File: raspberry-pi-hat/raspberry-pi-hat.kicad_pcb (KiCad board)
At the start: 2 copper layers, 58.5 x 66.5 mm, 31 parts, among them J1 IR_IN_JACK, J2 IR_OUT_JACK, J3 ADC0_JACK, J4 ADC1_JACK, J5 IR_IN_JMP, J6 IR_OUT_JMP, P1 RPi-GPIO, Q1 IRLML2803TRPBF, U1 MCP3204, U2 74AC86

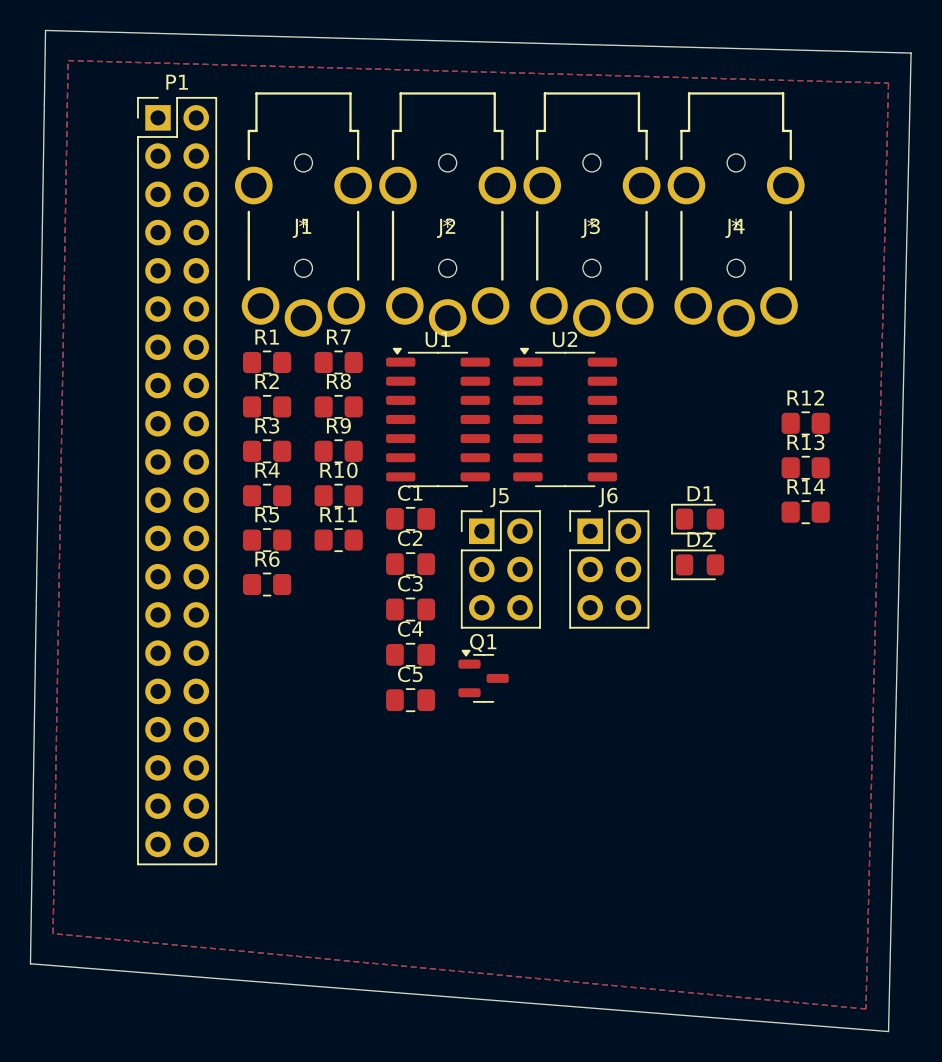
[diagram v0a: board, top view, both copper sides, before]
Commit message: pcb layout
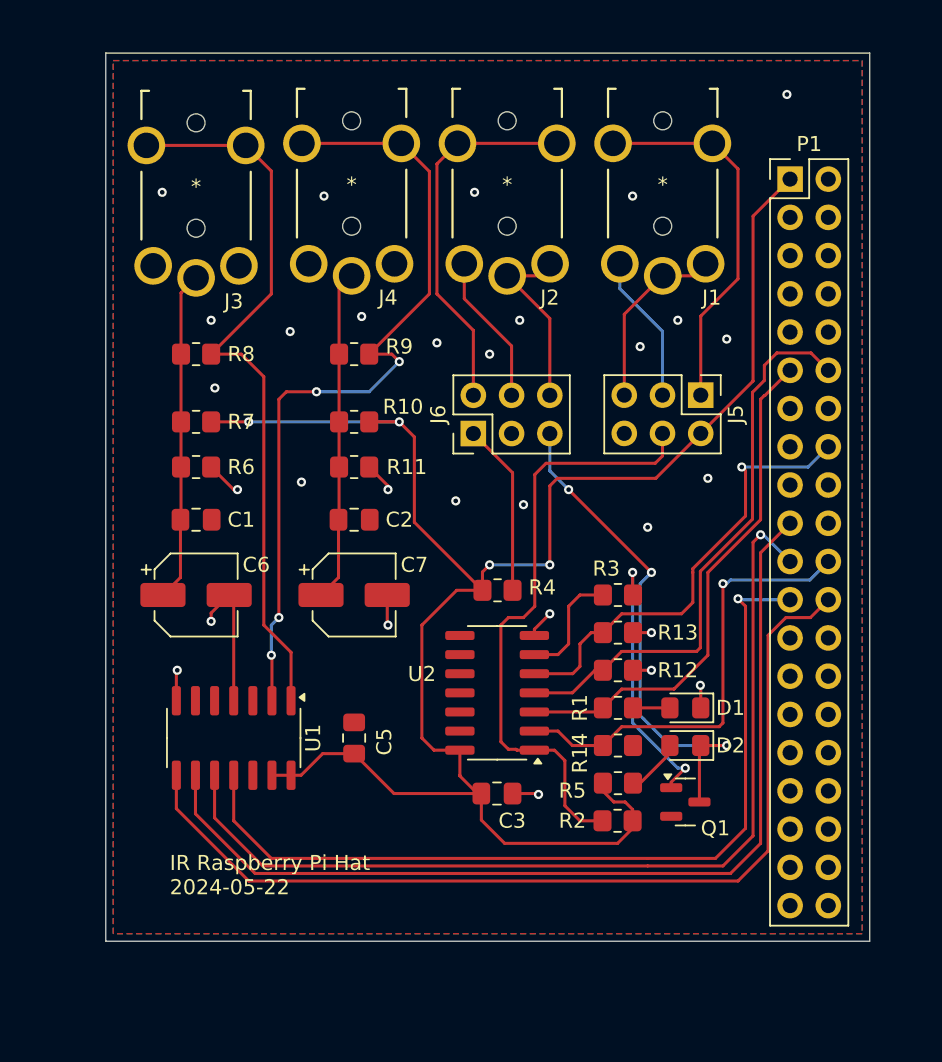
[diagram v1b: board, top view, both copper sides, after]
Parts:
- removed C4: 0.1uF, Capacitor_SMD:C_0805_2012Metric_Pad1.18x1.45mm_HandSolder
- added C6: 100uF, Capacitor_SMD:CP_Elec_5x5.3, F.Cu at (53.5, 86.5)
- added C7: 100uF, Capacitor_SMD:CP_Elec_5x5.3, F.Cu at (64.0, 86.5)
- moved P1 42.2 mm to (93.0, 58.9)
- moved R2 36.0 mm to (81.5, 101.5), turned to 180 degrees
- moved R1 32.7 mm to (81.5, 94.0)
- moved R5 28.4 mm to (81.5, 99.0), turned to 180 degrees
- moved J3 26.4 mm to (53.5, 59.4)
- moved J4 25.7 mm to (63.8, 59.2)
- moved R3 25.2 mm to (81.5, 86.5)
- moved U1 25.1 mm to (56.0, 96.0), turned to -90 degrees
- moved J1 24.0 mm to (84.5, 59.2)
- moved R12 20.6 mm to (81.5, 91.5), turned to 180 degrees
- moved R14 19.9 mm to (81.5, 96.5), turned to 180 degrees
- moved U2 18.7 mm to (73.5, 93.0), turned to 180 degrees
- moved J5 17.1 mm to (87.0, 73.2), turned to -90 degrees
- moved R13 16.6 mm to (81.5, 89.0), turned to 180 degrees
- moved R4 16.5 mm to (73.5, 86.2), turned to 180 degrees
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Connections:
- C1 pad 2: <NO NET> -> GND
- C2 pad 2: <NO NET> -> GND
- C3 pad 2: <NO NET> -> GND
- C5 pad 2: <NO NET> -> GND
- D1 pad 1: <NO NET> -> GND
- J1 pad R2: Net-(J5-Pin_1) -> Net-(J5-Pin_5)
- J1 pad S: Net-(J5-Pin_1) -> Net-(J5-Pin_5)
- J1 pad T: Net-(J5-Pin_5) -> Net-(J5-Pin_1)
- J5 pad 6: <NO NET> -> GND
- J6 pad 3: Net-(D2-K) -> unconnected-(J6-Pin_3-Pad3)
- P1 pad 25: <NO NET> -> GND
- P1 pad 39: <NO NET> -> GND
- P1 pad 9: <NO NET> -> GND
- Q1 pad 2: <NO NET> -> GND
- R11 pad 1: <NO NET> -> GND
- R12 pad 1: <NO NET> -> GND
- R13 pad 1: <NO NET> -> GND
- R14 pad 1: <NO NET> -> GND
- R6 pad 1: <NO NET> -> GND
- U1 pad 12: <NO NET> -> GND
- U1 pad 3: <NO NET> -> GND
- U1 pad 4: <NO NET> -> GND
- U1 pad 7: <NO NET> -> GND
- U2 pad 10: <NO NET> -> GND
- U2 pad 12: <NO NET> -> GND
- U2 pad 13: <NO NET> -> GND
- U2 pad 7: <NO NET> -> GND
- U2 pad 9: <NO NET> -> GND
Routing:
- net +3.3V: track 0.00 -> 121.6 mm, vias 0 -> 4
- net /MOSI: track 0.00 -> 64.6 mm
- net /MISO: track 0.00 -> 63.7 mm, vias 0 -> 1
- net /ADC_CS: track 0.00 -> 63.6 mm
- net /SCLK: track 0.00 -> 57.8 mm, vias 0 -> 1
- net /ADC_CH1: track 0.00 -> 54.5 mm, vias 0 -> 4
- net /ADC_CH0: track 0.00 -> 49.2 mm
- net Net-(J5-Pin_4): track 0.00 -> 40.4 mm
- net /IR_OUT: track 0.00 -> 37.9 mm
- net /IR_IN: track 0.00 -> 34.3 mm
- net Net-(D2-K): track 0.00 -> 33.9 mm, vias 0 -> 3
- net /IR_IN_POL: track 0.00 -> 30.4 mm, vias 0 -> 1
- net /IR_OUT_POL: track 0.00 -> 30.2 mm, vias 0 -> 1
- net GND: track 0.00 -> 25.7 mm, vias 0 -> 30
- net Net-(J5-Pin_1): track 0.00 -> 25.1 mm
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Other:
- board size 58.5 x 66.5 mm -> 50.8 x 59 mm
- board text added: "IR Raspberry Pi Hat 2024-05-22"
